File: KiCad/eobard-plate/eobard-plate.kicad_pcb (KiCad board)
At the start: 2 copper layers, 119 x 109 mm, 19 parts

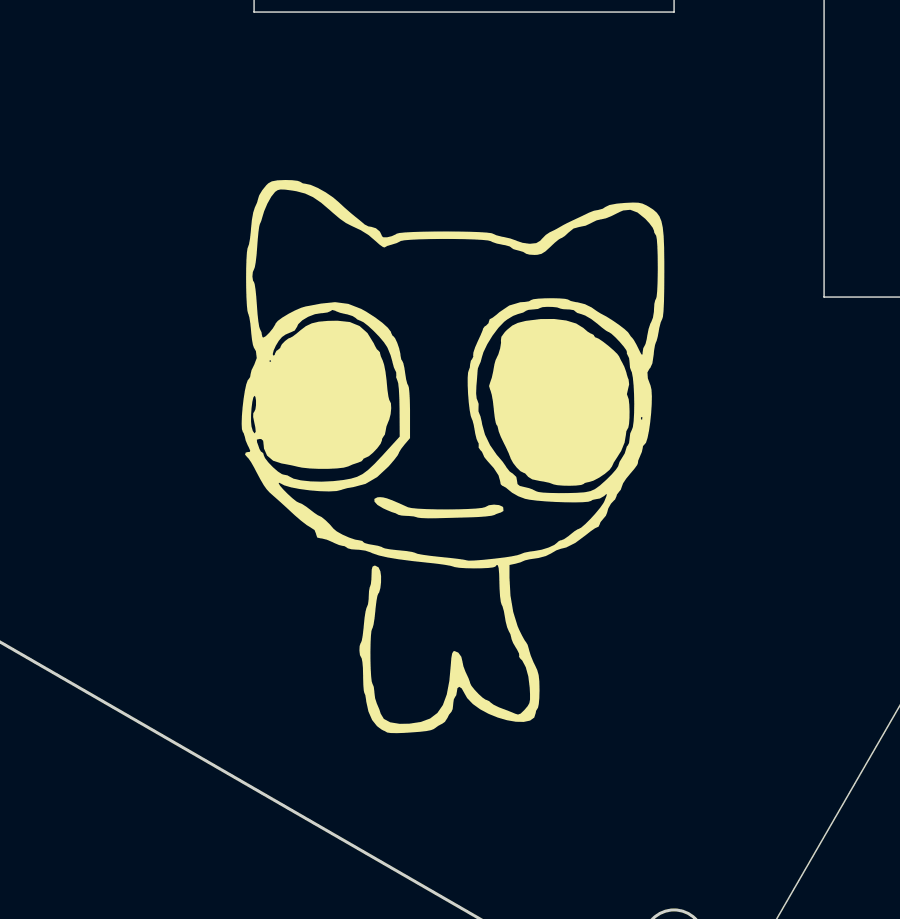
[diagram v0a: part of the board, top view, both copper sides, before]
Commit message: Updated KiCad Files
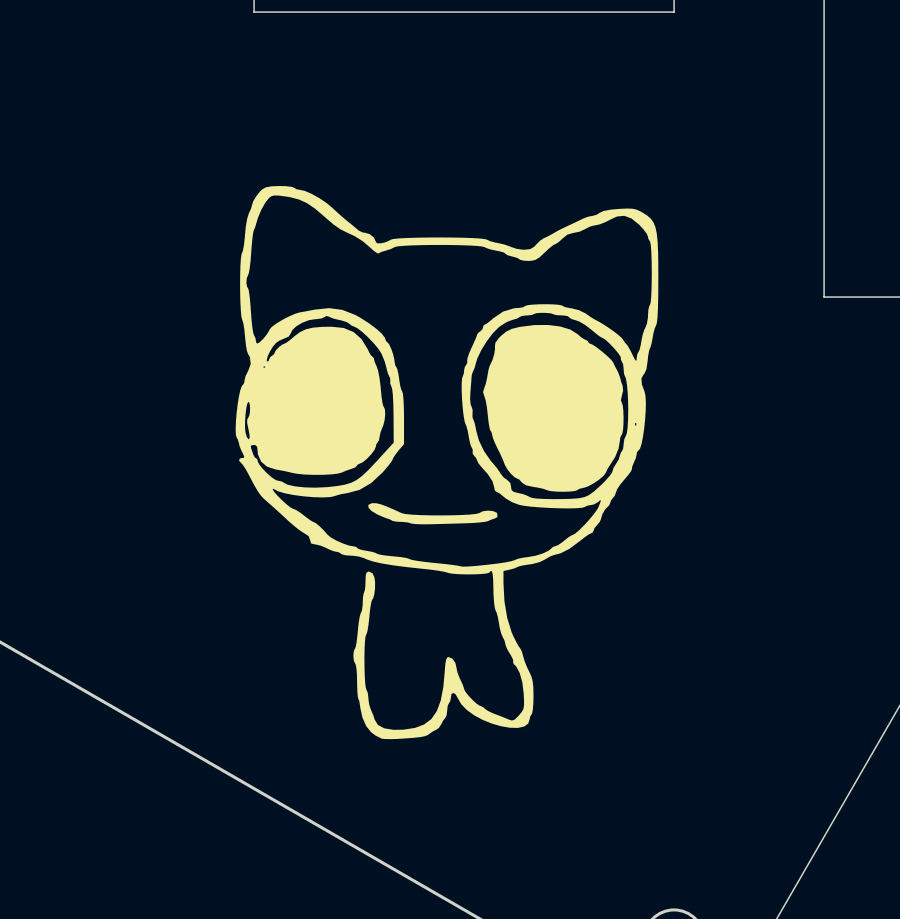
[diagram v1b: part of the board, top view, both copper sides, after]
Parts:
- moved G*** 0.28 mm to (147.0, 110.0)
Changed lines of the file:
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@@
   (title_block
     (title "Eobard Split Keyboard")
-    (date "2023-12-10")
-    (rev "2.2")
+    (date "2024-01-08")
+    (rev "1.1")
     (company "by viniciusbrit")
   )
@@
   )
   (footprint "Eobard-SVG-Files:ADHD-Creature" (layer "F.Cu")
-    (at 147.2 109.8)
+    (at 147 110)
     (attr board_only exclude_from_pos_files exclude_from_bom)
     (fp_text reference "G***" (at 0 -8.128) (layer "F.SilkS") hide
